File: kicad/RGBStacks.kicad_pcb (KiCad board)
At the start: 2 copper layers, 68.6 x 50.2 mm, 31 parts, among them J1 RJ45_8, J2 CONN_01X06, J3 CONN_02X12, J4 CONN_02X04, U1 PIC12F1572, U2 PIC12F1572, U3 PIC12F1572, U4 PIC12F1572, U5 ULN2003A, U6 ULN2003A

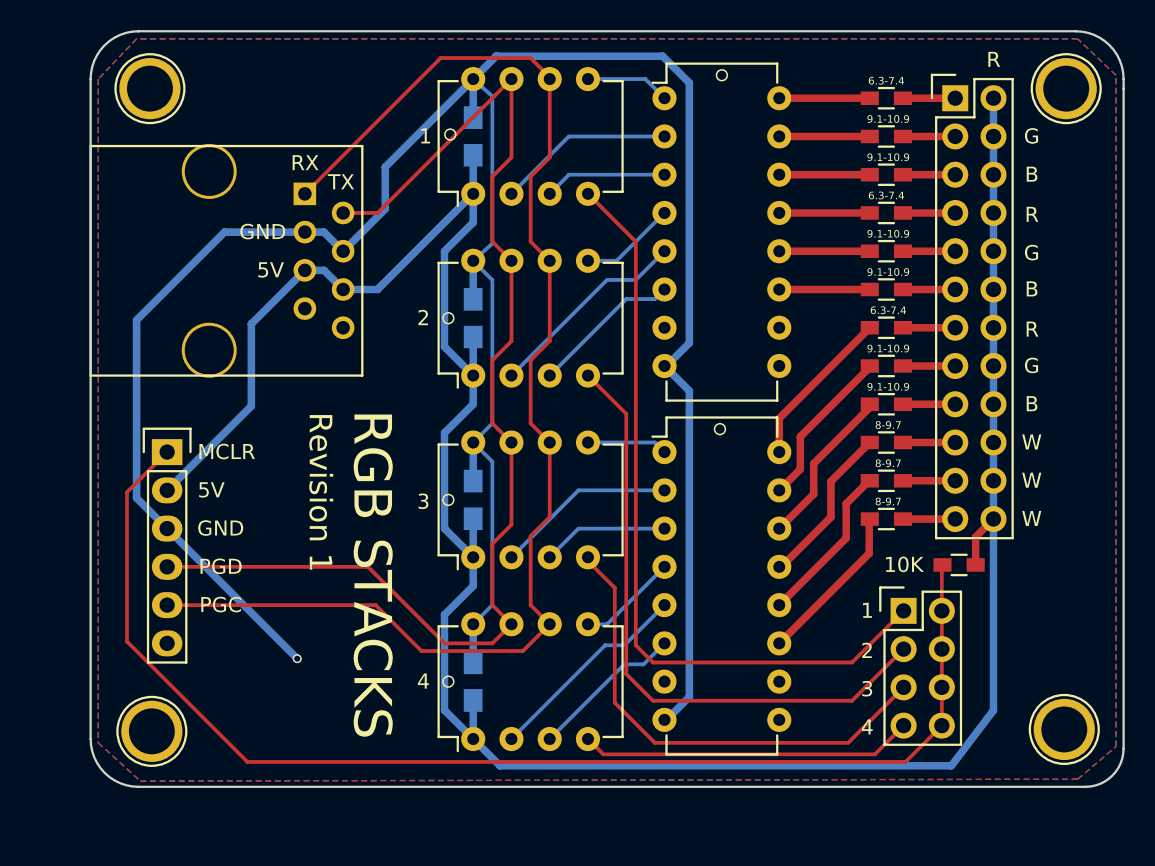
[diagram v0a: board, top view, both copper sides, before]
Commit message: Updated PCB.
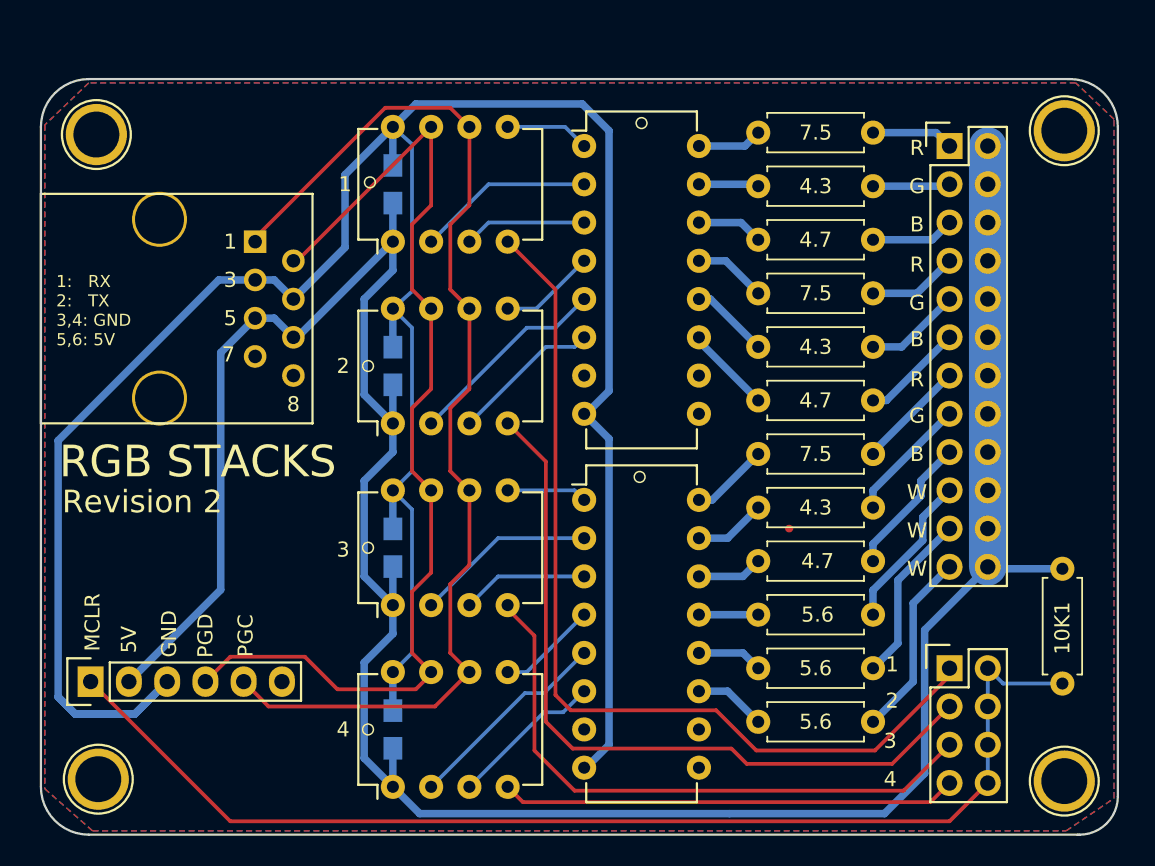
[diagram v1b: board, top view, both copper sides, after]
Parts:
- removed 10K, R10, R11, R12, R13, R2, R3, R4, R5, R6, R7, R8, R9: R, Resistors_SMD:R_0603_HandSoldering
- added 10K1: R, Resistors_THT:R_Axial_DIN0207_L6.3mm_D2.5mm_P7.62mm_Horizontal, F.Cu at (180.1, 109.3)
- added 4.3: R, Resistors_THT:R_Axial_DIN0207_L6.3mm_D2.5mm_P7.62mm_Horizontal, F.Cu at (167.5, 83.9)
- added 4.3: R, Resistors_THT:R_Axial_DIN0207_L6.3mm_D2.5mm_P7.62mm_Horizontal, F.Cu at (167.5, 94.6)
- added 4.3: R, Resistors_THT:R_Axial_DIN0207_L6.3mm_D2.5mm_P7.62mm_Horizontal, F.Cu at (167.5, 105.3)
- added 4.7: R, Resistors_THT:R_Axial_DIN0207_L6.3mm_D2.5mm_P7.62mm_Horizontal, F.Cu at (167.5, 87.5)
- added 4.7: R, Resistors_THT:R_Axial_DIN0207_L6.3mm_D2.5mm_P7.62mm_Horizontal, F.Cu at (167.5, 98.2)
- added 4.7: R, Resistors_THT:R_Axial_DIN0207_L6.3mm_D2.5mm_P7.62mm_Horizontal, F.Cu at (167.5, 108.8)
- added 5.6: R, Resistors_THT:R_Axial_DIN0207_L6.3mm_D2.5mm_P7.62mm_Horizontal, F.Cu at (167.5, 112.4)
- added 5.6: R, Resistors_THT:R_Axial_DIN0207_L6.3mm_D2.5mm_P7.62mm_Horizontal, F.Cu at (167.5, 116.0)
- added 5.6: R, Resistors_THT:R_Axial_DIN0207_L6.3mm_D2.5mm_P7.62mm_Horizontal, F.Cu at (167.5, 119.5)
- added 7.5: R, Resistors_THT:R_Axial_DIN0207_L6.3mm_D2.5mm_P7.62mm_Horizontal, F.Cu at (167.5, 80.4)
- added 7.5: R, Resistors_THT:R_Axial_DIN0207_L6.3mm_D2.5mm_P7.62mm_Horizontal, F.Cu at (167.5, 91.1)
- added 7.5: R, Resistors_THT:R_Axial_DIN0207_L6.3mm_D2.5mm_P7.62mm_Horizontal, F.Cu at (167.5, 101.7)
- moved J2 16.1 mm to (115.6, 116.8), turned to 90 degrees
- moved C1 6.21 mm to (135.6, 95.9)
- moved U3 6.21 mm to (135.6, 111.8)
- moved C2 6.21 mm to (135.6, 120.0)
- moved C3 6.21 mm to (135.6, 108.0)
- moved C4 6.21 mm to (135.6, 83.8)
- moved U1 6.21 mm to (135.6, 87.6)
- moved U2 6.21 mm to (135.6, 99.7)
- moved U4 6.21 mm to (135.6, 123.8)
- moved U6 6.21 mm to (148.3, 104.8)
- moved U5 6.21 mm to (148.3, 81.3)
- moved J4 4.88 mm to (172.6, 116.0)
- moved REF** 4.77 mm to (116.1, 123.3)
- moved REF** 4.68 mm to (116.0, 80.5)
- moved J1 4.58 mm to (120.1, 92.1)
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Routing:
- net RX/PGC: track 87.4 -> 74.7 mm
- net +5V: track 165.3 -> 176.9 mm
- net MCLR1: track 51.0 -> 61.7 mm
- net GND: track 168.4 -> 179.0 mm, vias 1 -> 0
- net TX/PGD: track 79.7 -> 69.3 mm
- net MCLR2: track 41.4 -> 50.4 mm
- net Net-(J3-Pad23): track 3.47 -> 12.4 mm
- net MCLR4: track 22.2 -> 30.3 mm
- net MCLR3: track 32.2 -> 40.3 mm
- net Net-(J3-Pad21): track 3.47 -> 11.4 mm
- net Net-(J3-Pad19): track 3.47 -> 10.4 mm
- net Net-(R11-Pad2): track 10.8 -> 4.06 mm
- net Net-(R12-Pad2): track 10.8 -> 4.36 mm
- net Net-(R10-Pad2): track 10.7 -> 4.36 mm
- net Net-(R9-Pad2): track 10.7 -> 4.78 mm
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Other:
- board size 68.6 x 50.2 mm -> 71.5 x 50.2 mm
- net class MaxCurrent added: clearance 0.2, trace_width 2.5, via_dia 0.6, via_drill 0.4
- board text added: "1: RX 2: TX 3,4: GND 5,6: 5V"
- board text added: "5"
- board text added: "7"
- board text added: "8"
- board text added: "Revision 2"
- board text removed: "6.3-7.4"
- board text removed: "8-9.7"
- board text removed: "9.1-10.9"
- board text removed: "RX"
- board text removed: "Revision 1"
- board text removed: "TX"
